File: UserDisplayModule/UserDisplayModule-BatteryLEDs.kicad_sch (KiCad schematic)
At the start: 17 parts, among them U5 74HC595

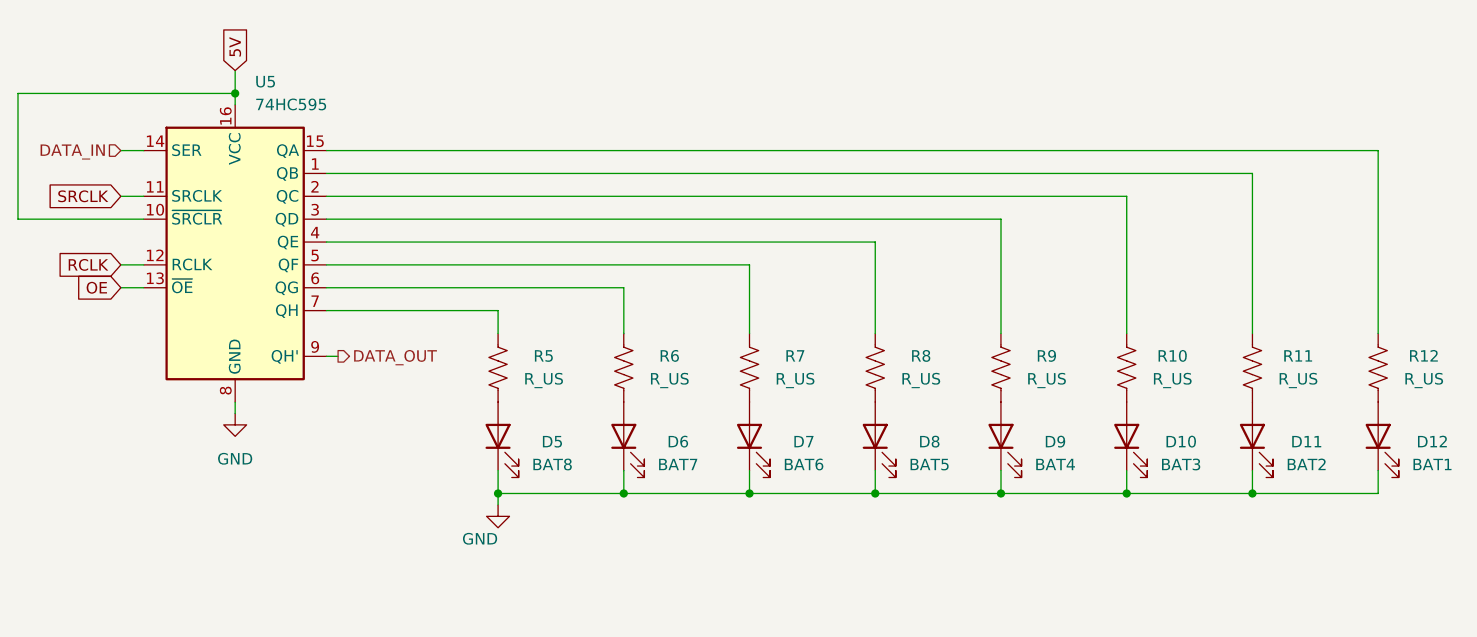
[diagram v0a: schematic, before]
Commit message: doubled LEDs + started PCB
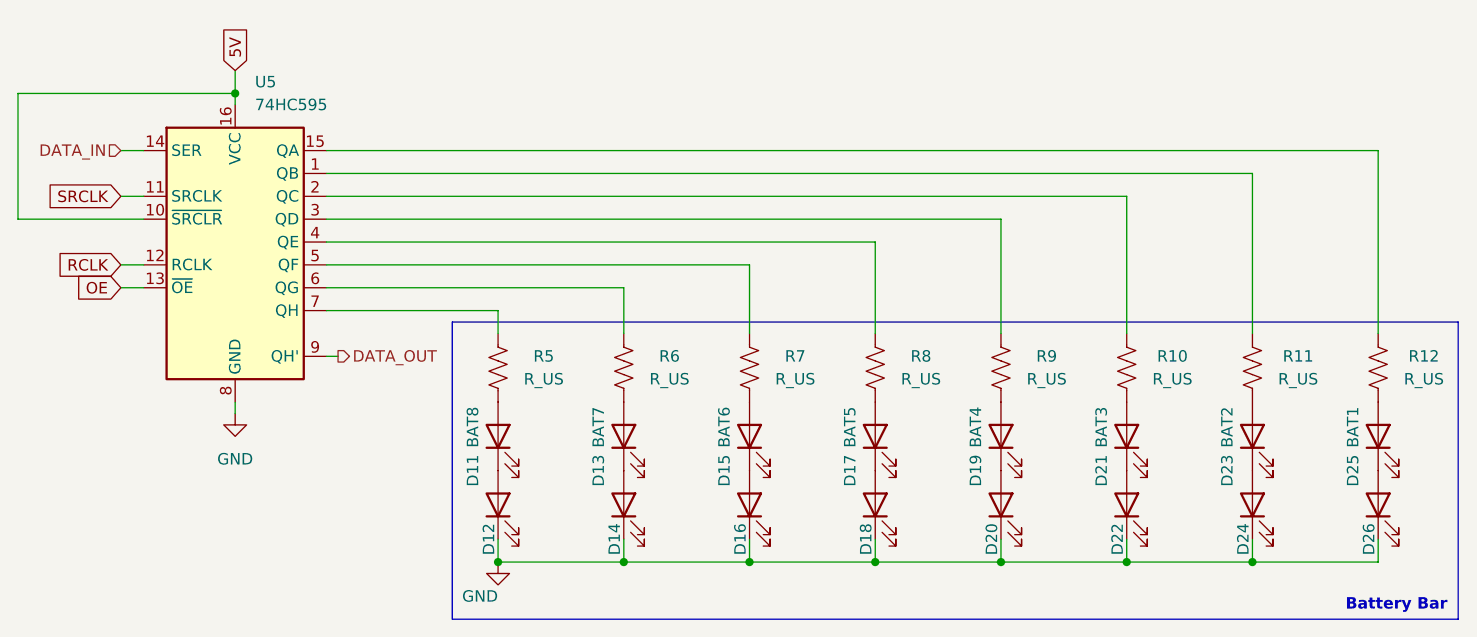
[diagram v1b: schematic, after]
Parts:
- removed D10: BAT3, symbol Device:LED
- removed D5: BAT8, symbol Device:LED
- removed D6: BAT7, symbol Device:LED
- removed D7: BAT6, symbol Device:LED
- removed D8: BAT5, symbol Device:LED
- removed D9: BAT4, symbol Device:LED
- added D13: BAT7, LED_SMD:LED_0805_2012Metric, symbol Device:LED
- added D14, D16, D18, D20, D22, D24, D25, D26: BAT1, LED_SMD:LED_0805_2012Metric, symbol Device:LED
- added D15: BAT6, LED_SMD:LED_0805_2012Metric, symbol Device:LED
- added D17: BAT5, LED_SMD:LED_0805_2012Metric, symbol Device:LED
- added D19: BAT4, LED_SMD:LED_0805_2012Metric, symbol Device:LED
- added D21: BAT3, LED_SMD:LED_0805_2012Metric, symbol Device:LED
- added D23: BAT2, LED_SMD:LED_0805_2012Metric, symbol Device:LED
- D11: value BAT2 -> BAT8; footprint (none) -> LED_SMD:LED_0805_2012Metric
- D12: footprint (none) -> LED_SMD:LED_0805_2012Metric
- R10, R11, R12, R5, R6, R7, R8, R9: footprint (none) -> Resistor_SMD:R_0805_2012Metric
- U5: footprint (none) -> ImportedFootprints:CD74HC595E
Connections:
- net GND: now also D14.1 (K), D16.1 (K), D18.1 (K), D20.1 (K), D22.1 (K), D24.1 (K), D26.1 (K); no longer D11.1 (K)
- net at R10.2: now also D21.2 (A)
- net at R6.2: now also D13.2 (A)
- net at R5.2: now also D11.2 (A)
- net at R7.2: now also D15.2 (A)
- net at R9.2: now also D19.2 (A)
- net at R8.2: now also D17.2 (A)
- net at D12.2 (A): now also D11.1 (K); no longer R12.2
- net at R11.2: now also D23.2 (A); no longer D11.2 (A)
- new net: D21.1 (K), D22.2 (A)
- new net: D13.1 (K), D14.2 (A)
- new net: D25.1 (K), D26.2 (A)
- new net: D19.1 (K), D20.2 (A)
- new net: D17.1 (K), D18.2 (A)
- new net: D23.1 (K), D24.2 (A)
- new net: D15.1 (K), D16.2 (A)
- new net: D25.2 (A), R12.2
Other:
- note added: "Battery Bar"
